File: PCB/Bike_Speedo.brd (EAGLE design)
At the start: 70.9 x 67.8 mm, 28 parts, among them IC2 TPS61202, J1 TE_CONNECTIVITY_1981568-1TE_C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, P1 BAT, U1 MICROCHIP_MCP73833-AMI-UNMICR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, U2 NUCLEO-F446RE

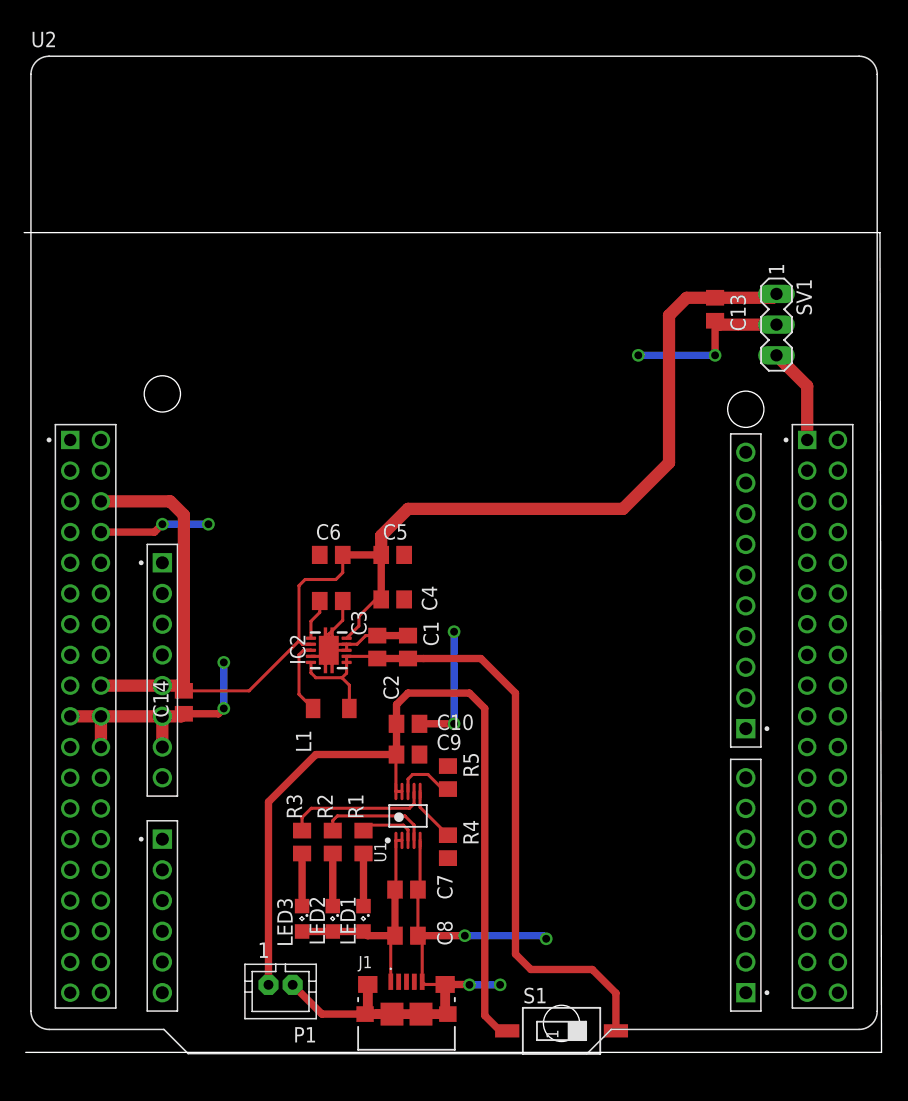
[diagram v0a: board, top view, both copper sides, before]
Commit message: modified PCB
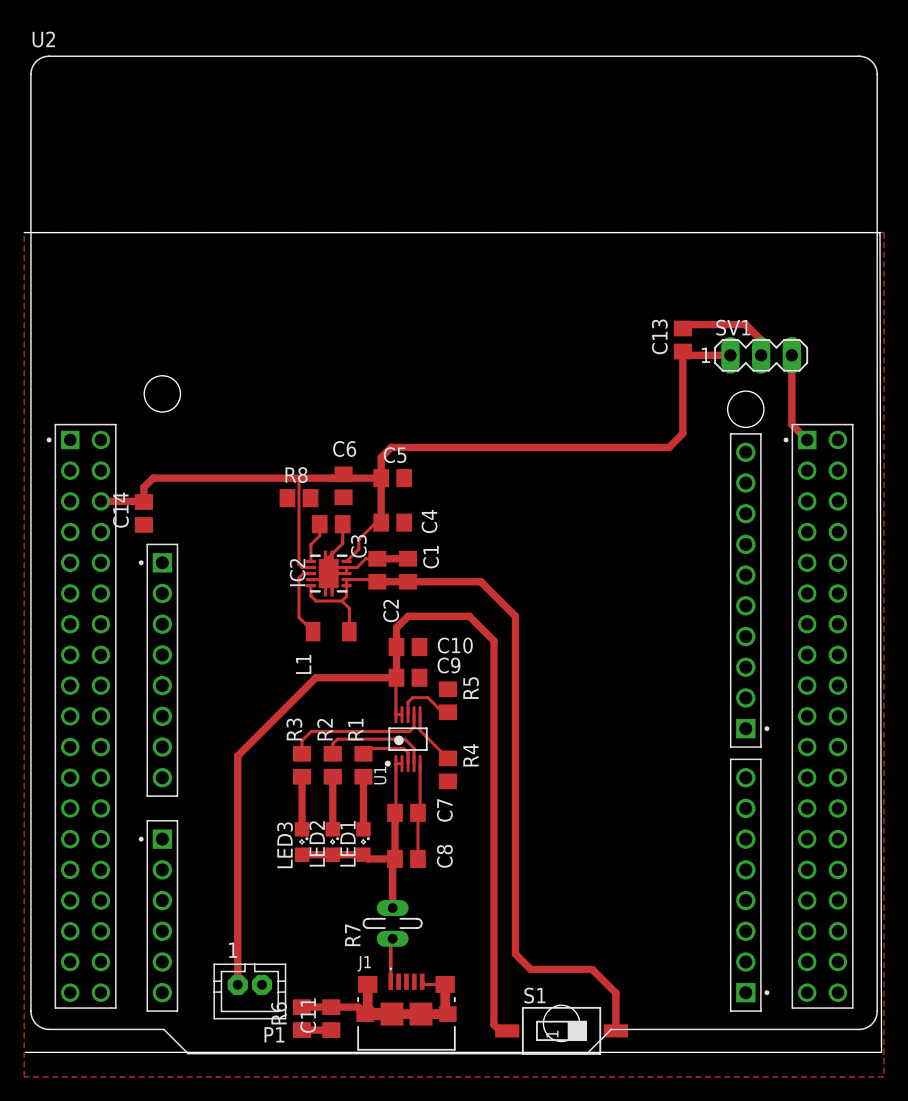
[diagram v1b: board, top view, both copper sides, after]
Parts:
- added C11: 10pF, rcl:C0805
- added R6: 1Meg, rcl:R0805
- added R7: (no value), ptc-ntc:P660
- added R8: 0R, rcl:R0805
- moved C14 16.0 mm to (130.6, 47.9)
- moved C1 6.35 mm to (152.4, 43.2)
- moved C2 6.35 mm to (149.9, 43.2)
- moved C3 6.35 mm to (146.1, 47.0)
- moved C7 6.35 mm to (152.3, 23.1)
- moved L1 6.35 mm to (146.1, 38.1)
- moved R4 6.35 mm to (155.7, 26.7)
- moved U1 6.35 mm to (152.4, 29.2)
- moved LED1 6.35 mm to (148.7, 20.7)
- moved LED2 6.35 mm to (146.2, 20.7)
- moved LED3 6.35 mm to (143.6, 20.7)
- moved C10 6.35 mm to (152.4, 36.8)
- moved C8 6.35 mm to (152.3, 19.3)
- moved C9 6.35 mm to (152.4, 34.3)
- moved R1 6.35 mm to (148.7, 27.1)
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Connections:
- new net CN6_+5V: U2.CN6_5
- new net CN7_+5V: U2.CN7_18
- new net N$1: J1.1, R7.1
- new net N$5: C11.2, J1.10, J1.11, J1.5, J1.6, J1.7, J1.8, J1.9, R6.2
- net +5V: no longer U2.CN6_5, U2.CN7_18
- net GND: now also C11.1, R6.1, R8.1, R8.2; no longer J1.10, J1.11, J1.5, J1.6, J1.7, J1.8, J1.9
- net N$4: now also R7.2; no longer J1.1
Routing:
- net GND: track 122.0 -> 34.8 mm, vias 12 -> 0
- net +5V: track 112.6 -> 80.3 mm
- net N$5: track 0.00 -> 19.7 mm
- net N$15: track 71.0 -> 84.8 mm
- net V_BAT: track 58.3 -> 64.4 mm
- net N$1: track 0.00 -> 3.62 mm
- net SIGNAL_SENSOR: track 8.05 -> 7.53 mm
- added copper zone on layer 1, net GND

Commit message: Update schematic and board
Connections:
- removed net LCD_BL: U2.CN5_2
- removed net LCD_CS: U2.CN5_3
- removed net LCD_DC: U2.CN9_8
- removed net LCD_RST: U2.CN5_1
- removed net MISO: U2.CN5_5
- removed net MOSI: U2.CN5_4
- removed net RESET: U2.CN6_3
- removed net SCLK: U2.CN5_6
- removed net TP_BUSY: U2.CN9_7
- removed net TP_CS: U2.CN9_5
- removed net TP_IRQ: U2.CN9_4
- new net CN5_GND: U2.CN5_7
- new net CN6_GND: U2.CN6_6, U2.CN6_7
- net GND: no longer U2.CN5_7, U2.CN6_6, U2.CN6_7
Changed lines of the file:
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@@
 <contactref element="P1" pad="2"/>
 <contactref element="SV1" pad="2"/>
-<contactref element="U2" pad="CN5_7"/>
 <contactref element="U2" pad="CN10_9"/>
 <contactref element="U2" pad="CN10_20"/>
@@
 <wire x1="180.34" y1="63.5" x2="181.61" y2="62.23" width="0.6096" layer="1"/>
 <wire x1="181.61" y1="62.23" x2="181.61" y2="60.96" width="0.6096" layer="1"/>
-<contactref element="U2" pad="CN6_7"/>
-<contactref element="U2" pad="CN6_6"/>
 <polygon width="0.6096" layer="1">
 <vertex x="120.65" y="71.12"/>
@@
 <vertex x="120.65" y="1.27"/>
 </polygon>
+<wire x1="185.42" y1="43.8" x2="181.61" y2="60.96" width="0" layer="19" extent="1-1"/>
+<wire x1="187.96" y1="31.1" x2="185.42" y2="43.8" width="0" layer="19" extent="1-1"/>
+<wire x1="152.08" y1="50.8" x2="175.133" y2="63.18" width="0" layer="19" extent="1-1"/>
+<wire x1="152.08" y1="47.117" x2="152.08" y2="50.8" width="0" layer="19" extent="1-1"/>
+<wire x1="152.4" y1="44.13" x2="152.08" y2="47.117" width="0" layer="19" extent="1-1"/>
+<wire x1="145.845" y1="42.91" x2="146.12" y2="42.91" width="0" layer="19" extent="1-1"/>
+<wire x1="145.57" y1="42.91" x2="145.845" y2="42.91" width="0" layer="19" extent="1-1"/>
+<wire x1="147.066" y1="49.215" x2="147" y2="46.99" width="0" layer="19" extent="1-1"/>
+<wire x1="144.333" y1="49.149" x2="147.066" y2="49.215" width="0" layer="19" extent="1-1"/>
+<wire x1="142.433" y1="49.149" x2="144.333" y2="49.149" width="0" layer="19" extent="1-1"/>
+<wire x1="153.35" y1="36.83" x2="152.4" y2="44.13" width="0" layer="19" extent="1-1"/>
+<wire x1="153.35" y1="34.29" x2="153.35" y2="36.83" width="0" layer="19" extent="1-1"/>
+<wire x1="155.702" y1="33.335" x2="153.35" y2="34.29" width="0" layer="19" extent="1-1"/>
+<wire x1="153.4" y1="27.185" x2="155.702" y2="33.335" width="0" layer="19" extent="1-1"/>
+<wire x1="155.702" y1="25.72" x2="153.4" y2="27.185" width="0" layer="19" extent="1-1"/>
+<wire x1="130.556" y1="46.929" x2="142.433" y2="49.149" width="0" layer="19" extent="1-1"/>
+<wire x1="127" y1="46.34" x2="130.556" y2="46.929" width="0" layer="19" extent="1-1"/>
+<wire x1="127" y1="31.1" x2="127" y2="46.34" width="0" layer="19" extent="1-1"/>
+<wire x1="124.46" y1="31.1" x2="127" y2="31.1" width="0" layer="19" extent="1-1"/>
+<wire x1="127" y1="28.56" x2="127" y2="31.1" width="0" layer="19" extent="1-1"/>
+<wire x1="146.05" y1="5.146" x2="153.223" y2="19.304" width="0" layer="19" extent="1-1"/>
+<wire x1="140.319" y1="8.89" x2="143.637" y2="5.146" width="0" layer="19" extent="1-1"/>
 </signal>
 <signal name="VDD">
@@
 <wire x1="184.15" y1="55.23" x2="184.15" y2="60.96" width="0.6096" layer="1"/>
 </signal>
-<signal name="RESET">
-<contactref element="U2" pad="CN6_3"/>
-</signal>
-<signal name="TP_IRQ">
-<contactref element="U2" pad="CN9_4"/>
-</signal>
-<signal name="TP_CS">
-<contactref element="U2" pad="CN9_5"/>
-</signal>
-<signal name="TP_BUSY">
-<contactref element="U2" pad="CN9_7"/>
-</signal>
-<signal name="LCD_DC">
-<contactref element="U2" pad="CN9_8"/>
-</signal>
-<signal name="LCD_RST">
-<contactref element="U2" pad="CN5_1"/>
-</signal>
-<signal name="LCD_BL">
-<contactref element="U2" pad="CN5_2"/>
-</signal>
-<signal name="LCD_CS">
-<contactref element="U2" pad="CN5_3"/>
-</signal>
-<signal name="MOSI">
-<contactref element="U2" pad="CN5_4"/>
-</signal>
-<signal name="MISO">
-<contactref element="U2" pad="CN5_5"/>
-</signal>
-<signal name="SCLK">
-<contactref element="U2" pad="CN5_6"/>
-</signal>
 <signal name="N$5">
 <contactref element="C11" pad="2"/>
@@
 <contactref element="U2" pad="CN6_5"/>
 </signal>
+<signal name="CN5_GND">
+<contactref element="U2" pad="CN5_7"/>
+</signal>
+<signal name="CN6_GND">
+<contactref element="U2" pad="CN6_6"/>
+<contactref element="U2" pad="CN6_7"/>
+<wire x1="132.08" y1="28.56" x2="132.08" y2="31.1" width="0" layer="19" extent="1-1"/>
+</signal>
 </signals>
